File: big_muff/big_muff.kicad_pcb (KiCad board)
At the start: 2 copper layers, 60 x 79 mm, 51 parts, among them J1 PJ-202A, J3 Conn_01x04_Socket, Q1 2N5088, Q2 2N5088, Q3 2N5088, Q4 2N5088

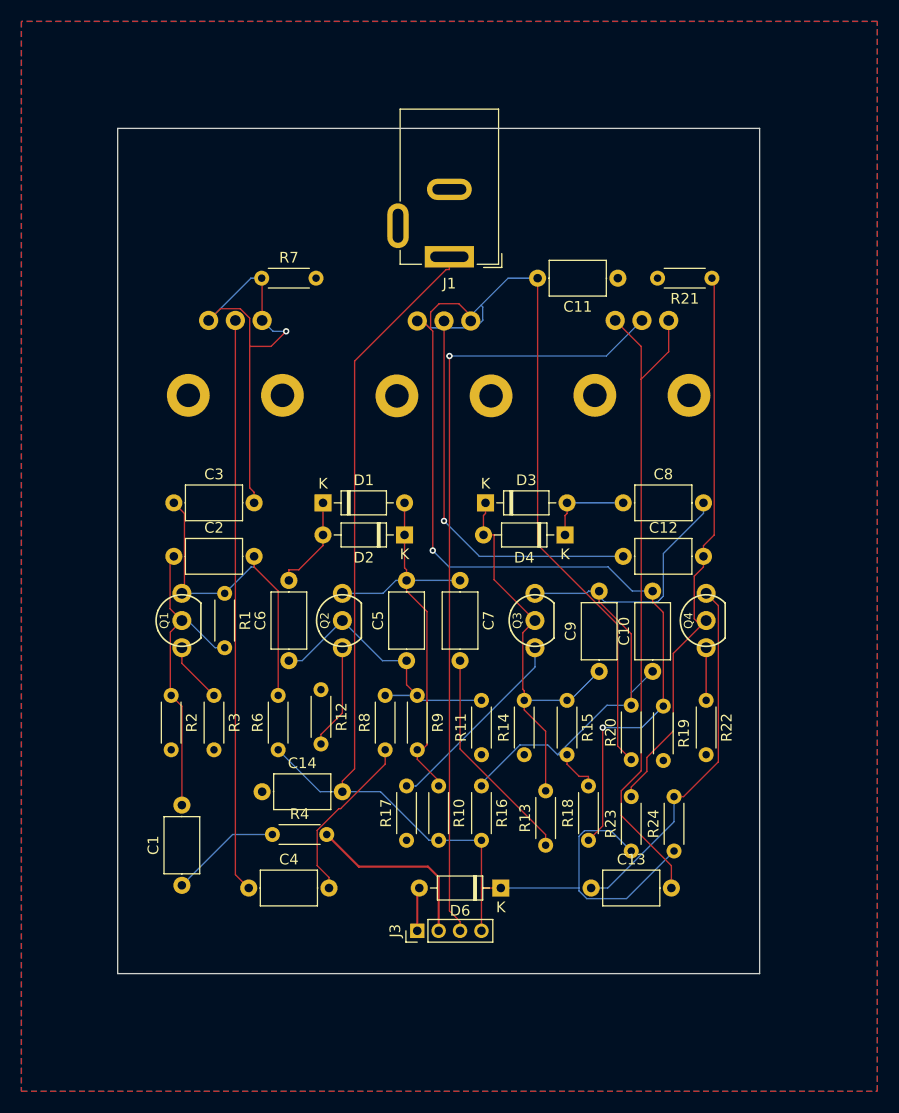
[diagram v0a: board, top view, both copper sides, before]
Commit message: Continue work with big muff
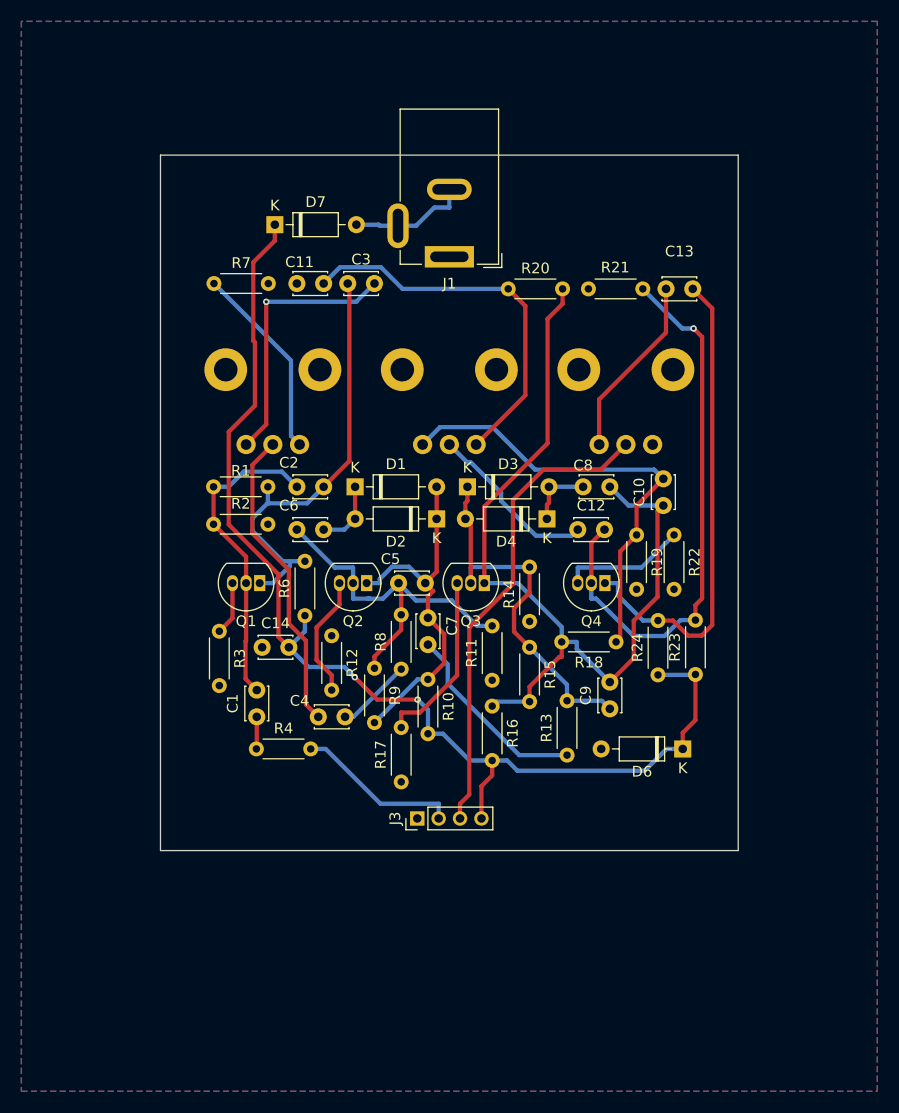
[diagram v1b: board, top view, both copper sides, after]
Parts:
- added D7: 1N4148, Diode_THT:D_DO-35_SOD27_P7.62mm_Horizontal, F.Cu at (143.7, 69.0)
- C1, C10, C11, C12, C13, C2, C3, C4, C5, C6, C7, C8, C9: footprint Capacitor_THT:C_Axial_L5.1mm_D3.1mm_P7.50mm_Horizontal -> Capacitor_THT:C_Disc_D3.0mm_W2.0mm_P2.50mm
- C14: value 0.1u -> 1u; footprint Capacitor_THT:C_Axial_L5.1mm_D3.1mm_P7.50mm_Horizontal -> Capacitor_THT:C_Disc_D3.0mm_W2.0mm_P2.50mm
- Q1, Q2, Q3, Q4: value 2N5088 -> BC550; footprint 2N5088:TO92 -> Package_TO_SOT_THT:TO-92_Inline
- R2: value 100k -> 47k
- moved C13 56.8 mm to (182.8, 75.0), turned to 180 degrees
- moved R20 45.5 mm to (165.5, 75.0), turned to 0 degrees
- moved C11 30.0 mm to (145.8, 74.5), turned to 0 degrees
- moved C3 26.2 mm to (150.5, 74.5)
- moved D6 21.4 mm to (181.8, 118.0)
- moved R18 18.7 mm to (175.6, 108.0), turned to 180 degrees
- moved R23 17.6 mm to (183.0, 111.0)
- moved C4 17.3 mm to (147.8, 115.0)
- moved C1 17.2 mm to (142.0, 115.0)
- moved R24 16.5 mm to (179.5, 111.1)
- moved R2 16.5 mm to (138.0, 97.0), turned to 0 degrees
- moved R19 16.2 mm to (177.5, 98.0)
- moved R22 15.7 mm to (181.0, 98.0)
- moved C10 15.5 mm to (180.0, 95.2)
- moved C14 13.5 mm to (142.5, 108.5)
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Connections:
- J1 pad 1: +9V -> GND
- J1 pad 2: GND -> Net-(D7-A)
- J1 pad 3: GND -> Net-(D7-A)
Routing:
- net Net-(C13-Pad2): track 63.3 -> 17.1 mm
- net Net-(C10-Pad2): track 80.0 -> 42.3 mm, vias 2 -> 0
- net Net-(C11-Pad2): track 65.3 -> 35.8 mm
- net Output: track 73.5 -> 44.5 mm, vias 1 -> 0
- net Net-(C4-Pad1): track 53.6 -> 28.8 mm
- net Net-(C12-Pad1): track 37.3 -> 16.2 mm, vias 1 -> 0
- net Net-(Q3-C): track 62.6 -> 82.2 mm
- net Net-(D7-A): track 0.00 -> 11.1 mm
- net Net-(Q4-C): track 34.4 -> 45.3 mm
- net Net-(C4-Pad2): track 16.1 -> 7.10 mm
- net Net-(Q1-C): track 31.7 -> 40.6 mm
- net +9V: track 116.4 -> 107.9 mm, vias 0 -> 2
- net Net-(R7-Pad1): track 10.6 -> 18.4 mm
- net Net-(C1-Pad1): track 10.4 -> 3.02 mm
- net Net-(Q2-B): track 27.0 -> 34.0 mm
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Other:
- board size 60 x 79 mm -> 54 x 65 mm
